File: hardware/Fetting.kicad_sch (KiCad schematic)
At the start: 5 parts, among them Q19 NMOS

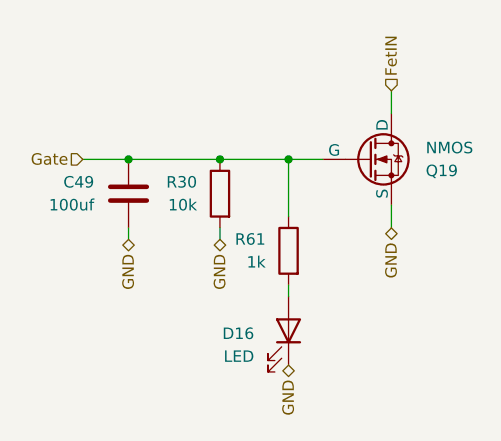
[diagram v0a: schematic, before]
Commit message: pedning review
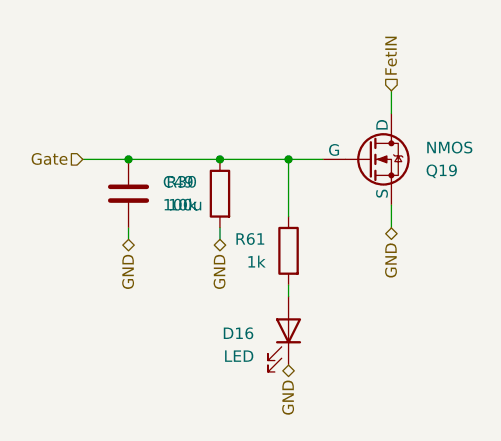
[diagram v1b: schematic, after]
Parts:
- C49: value 100uf -> 100u
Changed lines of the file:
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@@
 		(fields_autoplaced yes)
 		(property "Reference" "C49"
-			(at 110.49 82.5499 0)
+			(at 118.11 82.5499 0)
 			(show_name no)
 			(do_not_autoplace no)
@@
 					(size 1.27 1.27)
 				)
-				(justify left)
+				(justify right)
 			)
 		)
-		(property "Value" "100uf"
-			(at 110.49 85.0899 0)
+		(property "Value" "100u"
+			(at 118.11 85.0899 0)
 			(show_name no)
 			(do_not_autoplace no)
@@
 					(size 1.27 1.27)
 				)
-				(justify left)
+				(justify right)
 			)
 		)

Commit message: footprint! mising 2
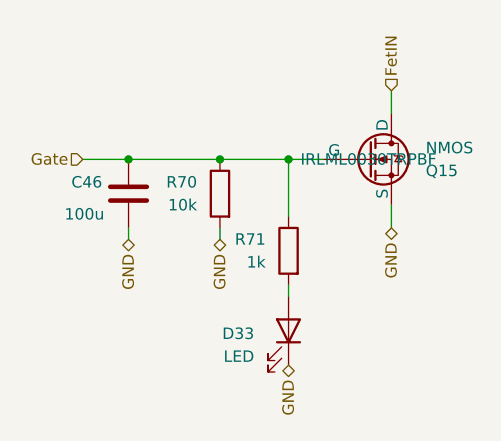
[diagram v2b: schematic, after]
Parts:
- C46: renamed from C49; footprint (none) -> Capacitor_SMD:C_0603_1608Metric_Pad1.08x0.95mm_HandSolder
- Q15: renamed from Q19; footprint (none) -> LSOM_IRLM:SOT23; p/n (none) -> IRLML0030TRPBF
- R70: renamed from R30; footprint (none) -> Resistor_SMD:R_0603_1608Metric_Pad0.98x0.95mm_HandSolder
- R71: renamed from R61; footprint (none) -> Resistor_SMD:R_0603_1608Metric_Pad0.98x0.95mm_HandSolder
- renumbered D16 to D33
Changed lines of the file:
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@@
 		(dnp no)
 		(fields_autoplaced yes)
-		(property "Reference" "R30"
+		(property "Reference" "R70"
 			(at 121.92 82.5499 0)
 			(show_name no)
@@
 			)
 		)
-		(property "Footprint" ""
+		(property "Footprint" "Resistor_SMD:R_0603_1608Metric_Pad0.98x0.95mm_HandSolder"
 			(at 126.238 83.82 90)
 			(hide yes)
@@
 			(project "DEI"
 				(path "/1469f349-54e5-4a37-953e-ac48c70e29b2/62c62208-3ad7-4747-b842-0db22efa2c00/b37209a4-58c6-485e-9ae0-dfc559dfc74c"
-					(reference "R30")
+					(reference "R70")
 					(unit 1)
 				)
 				(path "/1469f349-54e5-4a37-953e-ac48c70e29b2/62c62208-3ad7-4747-b842-0db22efa2c00/c5ef5451-f376-40f1-978e-9f58b1b49c9d"
-					(reference "R31")
+					(reference "R80")
 					(unit 1)
 				)
 				(path "/1469f349-54e5-4a37-953e-ac48c70e29b2/62c62208-3ad7-4747-b842-0db22efa2c00/d7551ab7-02b4-4db5-ad32-6a64598e5e63"
-					(reference "R32")
+					(reference "R82")
 					(unit 1)
 				)
@@
 		(in_pos_files yes)
 		(dnp no)
-		(property "Reference" "Q19"
+		(property "Reference" "Q15"
 			(at 147.32 81.2801 0)
 			(show_name no)
@@
 			)
 		)
-		(property "Footprint" ""
+		(property "Footprint" "LSOM_IRLM:SOT23"
 			(at 146.05 77.47 0)
 			(hide yes)
@@
 			(at 140.97 95.25 0)
 			(hide yes)
+			(show_name no)
+			(do_not_autoplace no)
+			(effects
+				(font
+					(size 1.27 1.27)
+				)
+			)
+		)
+		(property "p/n" "IRLML0030TRPBF"
+			(at 140.97 80.01 0)
 			(show_name no)
 			(do_not_autoplace no)
@@
 			(project "DEI"
 				(path "/1469f349-54e5-4a37-953e-ac48c70e29b2/62c62208-3ad7-4747-b842-0db22efa2c00/b37209a4-58c6-485e-9ae0-dfc559dfc74c"
-					(reference "Q19")
+					(reference "Q15")
 					(unit 1)
 				)
 				(path "/1469f349-54e5-4a37-953e-ac48c70e29b2/62c62208-3ad7-4747-b842-0db22efa2c00/c5ef5451-f376-40f1-978e-9f58b1b49c9d"
-					(reference "Q20")
+					(reference "Q16")
 					(unit 1)
 				)
 				(path "/1469f349-54e5-4a37-953e-ac48c70e29b2/62c62208-3ad7-4747-b842-0db22efa2c00/d7551ab7-02b4-4db5-ad32-6a64598e5e63"
-					(reference "Q21")
+					(reference "Q17")
 					(unit 1)
 				)
@@
 		(in_pos_files yes)
 		(dnp no)
-		(fields_autoplaced yes)
-		(property "Reference" "C49"
-			(at 118.11 82.5499 0)
+		(property "Reference" "C46"
+			(at 107.95 82.55 0)
 			(show_name no)
 			(do_not_autoplace no)
@@
 		)
 		(property "Value" "100u"
-			(at 118.11 85.0899 0)
+			(at 107.188 86.106 0)
 			(show_name no)
 			(do_not_autoplace no)
@@
 			)
 		)
-		(property "Footprint" ""
+		(property "Footprint" "Capacitor_SMD:C_0603_1608Metric_Pad1.08x0.95mm_HandSolder"
 			(at 113.3348 87.63 0)
 			(hide yes)
@@
 			(project "DEI"
 				(path "/1469f349-54e5-4a37-953e-ac48c70e29b2/62c62208-3ad7-4747-b842-0db22efa2c00/b37209a4-58c6-485e-9ae0-dfc559dfc74c"
-					(reference "C49")
+					(reference "C46")
 					(unit 1)
 				)
 				(path "/1469f349-54e5-4a37-953e-ac48c70e29b2/62c62208-3ad7-4747-b842-0db22efa2c00/c5ef5451-f376-40f1-978e-9f58b1b49c9d"
-					(reference "C60")
+					(reference "C61")
 					(unit 1)
 				)
 				(path "/1469f349-54e5-4a37-953e-ac48c70e29b2/62c62208-3ad7-4747-b842-0db22efa2c00/d7551ab7-02b4-4db5-ad32-6a64598e5e63"
-					(reference "C61")
+					(reference "C62")
 					(unit 1)
 				)
@@
 		(dnp no)
 		(fields_autoplaced yes)
-		(property "Reference" "D16"
+		(property "Reference" "D33"
 			(at 128.27 99.3774 90)
 			(show_name no)
@@
 			(project "DEI"
 				(path "/1469f349-54e5-4a37-953e-ac48c70e29b2/62c62208-3ad7-4747-b842-0db22efa2c00/b37209a4-58c6-485e-9ae0-dfc559dfc74c"
-					(reference "D16")
+					(reference "D33")
 					(unit 1)
 				)
 				(path "/1469f349-54e5-4a37-953e-ac48c70e29b2/62c62208-3ad7-4747-b842-0db22efa2c00/c5ef5451-f376-40f1-978e-9f58b1b49c9d"
-					(reference "D17")
+					(reference "D37")
 					(unit 1)
 				)
 				(path "/1469f349-54e5-4a37-953e-ac48c70e29b2/62c62208-3ad7-4747-b842-0db22efa2c00/d7551ab7-02b4-4db5-ad32-6a64598e5e63"
-					(reference "D19")
+					(reference "D38")
 					(unit 1)
 				)
@@
 		(dnp no)
 		(fields_autoplaced yes)
-		(property "Reference" "R61"
+		(property "Reference" "R71"
 			(at 129.54 88.8999 0)
 			(show_name no)
@@
 			)
 		)
-		(property "Footprint" ""
+		(property "Footprint" "Resistor_SMD:R_0603_1608Metric_Pad0.98x0.95mm_HandSolder"
 			(at 133.858 90.17 90)
 			(hide yes)
@@
 			(project "DEI"
 				(path "/1469f349-54e5-4a37-953e-ac48c70e29b2/62c62208-3ad7-4747-b842-0db22efa2c00/b37209a4-58c6-485e-9ae0-dfc559dfc74c"
-					(reference "R61")
+					(reference "R71")
 					(unit 1)
 				)
 				(path "/1469f349-54e5-4a37-953e-ac48c70e29b2/62c62208-3ad7-4747-b842-0db22efa2c00/c5ef5451-f376-40f1-978e-9f58b1b49c9d"
-					(reference "R70")
+					(reference "R81")
 					(unit 1)
 				)
 				(path "/1469f349-54e5-4a37-953e-ac48c70e29b2/62c62208-3ad7-4747-b842-0db22efa2c00/d7551ab7-02b4-4db5-ad32-6a64598e5e63"
-					(reference "R91")
-					(unit 1)
-				)
+					(reference "R83")
+					(unit 1)
+				)
